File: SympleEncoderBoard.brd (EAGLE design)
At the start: 50.8 x 50.8 mm, 31 parts, among them IC1 STM32F446RET6

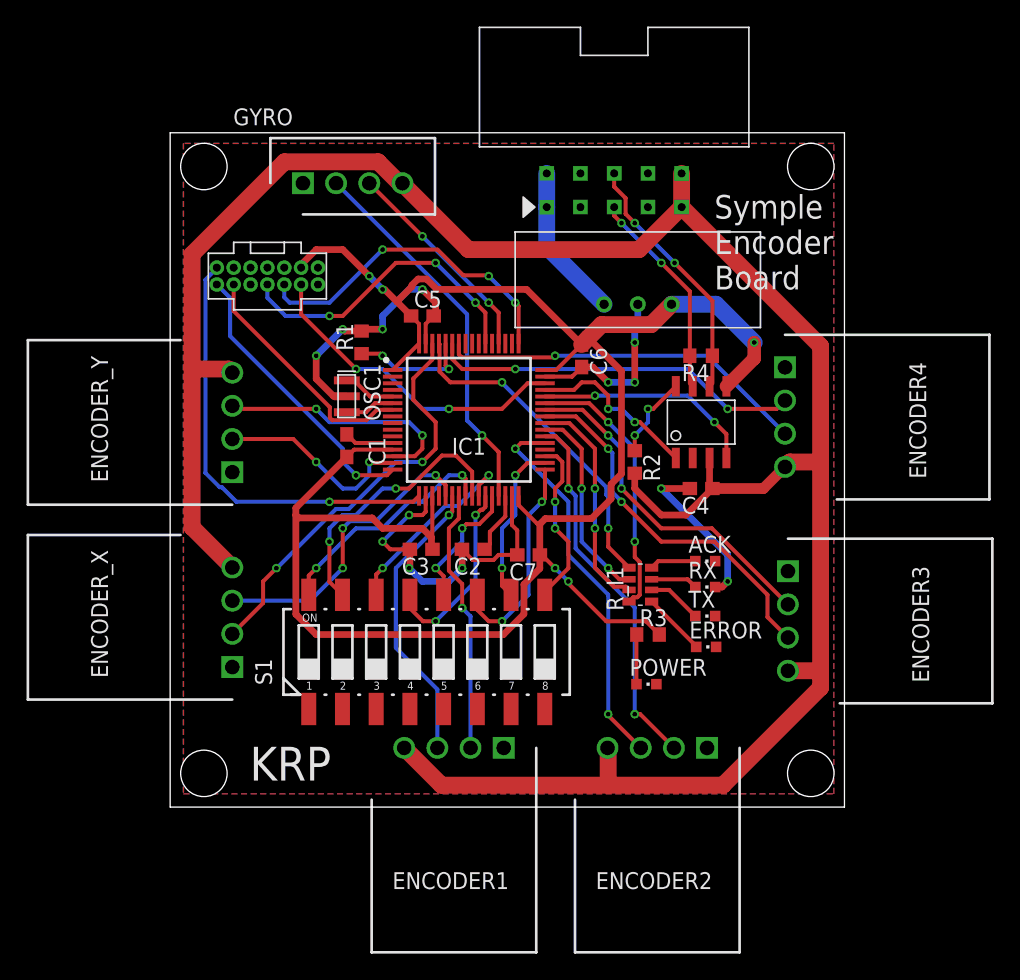
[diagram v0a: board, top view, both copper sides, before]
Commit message: エラー等修正しました。
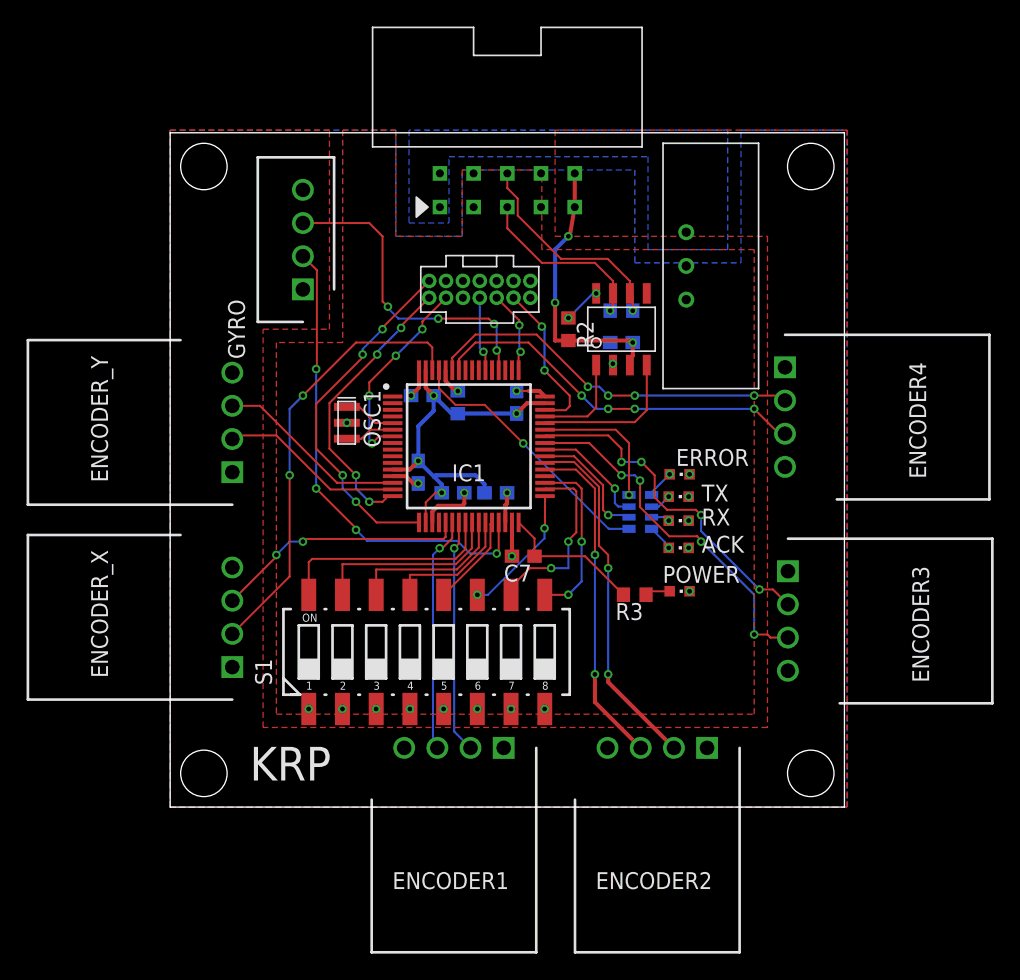
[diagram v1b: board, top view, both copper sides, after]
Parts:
- moved U$1 16.0 mm to (18.9, 40.7)
- moved ERROR 13.2 mm to (38.4, 25.1)
- moved C4 12.5 mm to (34.0, 35.0), flipped to the bottom, turned to 0 degrees
- moved R2 11.2 mm to (30.0, 36.0)
- moved TX 9.22 mm to (38.3, 23.4)
- moved U$3 9.22 mm to (34.0, 36.0)
- moved R1 8.54 mm to (21.7, 30.5), flipped to the bottom, turned to 270 degrees
- moved BOX10P-L1 8.05 mm to (25.4, 47.7)
- moved GYRO 8.00 mm to (10.0, 39.0), turned to 90 degrees
- moved POWER 7.43 mm to (38.4, 16.3)
- moved R4 6.90 mm to (34.0, 37.4), flipped to the bottom, turned to 0 degrees
- moved C6 6.02 mm to (26.1, 30.5), flipped to the bottom
- moved C5 6.00 mm to (19.0, 31.0), flipped to the bottom, turned to 180 degrees
- moved C1 5.74 mm to (18.7, 25.2), flipped to the bottom
- moved R_I1 5.48 mm to (35.4, 22.2), flipped to the bottom, turned to 270 degrees
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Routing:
- net +5V: track 175.9 -> 20.8 mm, vias 0 -> 3
- net +3.3V: track 149.0 -> 21.9 mm, vias 5 -> 4
- net GND: track 74.4 -> 32.6 mm, vias 13 -> 20
- net SWCLK: track 25.0 -> 6.26 mm, vias 3 -> 2
- net SWO: track 23.5 -> 5.63 mm, vias 3 -> 1
- net SWDIO: track 24.4 -> 11.9 mm
- net +12V: track 11.6 -> 0.00 mm
- net ERRORLED: track 20.4 -> 10.7 mm, vias 2 -> 1
- net LED1: track 16.8 -> 8.75 mm, vias 2 -> 1
- net I2C_SDA: track 16.1 -> 24.1 mm, vias 2 -> 4
- net I2C_SCL: track 28.6 -> 36.1 mm, vias 1 -> 4
- net N$1: track 9.08 -> 2.12 mm, vias 2 -> 1
- net SW7: track 20.8 -> 14.5 mm, vias 2 -> 0
- net VCP_RX: track 33.0 -> 26.8 mm, vias 1 -> 4
- net SW3: track 16.1 -> 10.0 mm
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- added copper zone on layer 16, net +12V
- added copper zone on layer 1, net +3.3V
- added copper zone on layer 1, net +5V
- removed copper zone on layer 1, net GND
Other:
- board text removed: "Symple Encoder Board"
